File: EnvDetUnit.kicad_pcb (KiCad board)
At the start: 2 copper layers, 36 x 10 mm, 19 parts, among them CN1 CON_GROVE, CN2 CON_GROVE, J1 Conn_01x03, J2 Conn_01x03, J3 Conn_01x02, U1 S89431

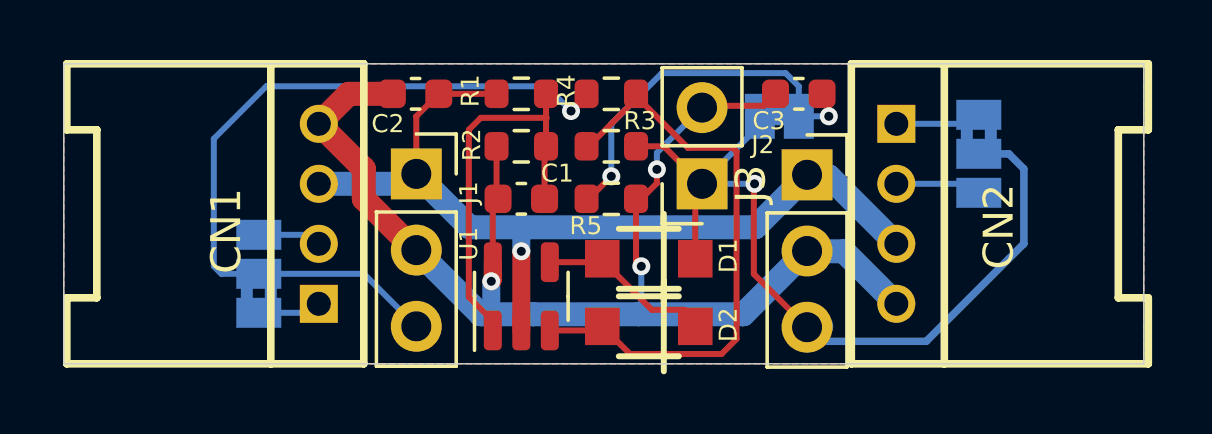
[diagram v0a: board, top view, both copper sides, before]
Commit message: update PCB data
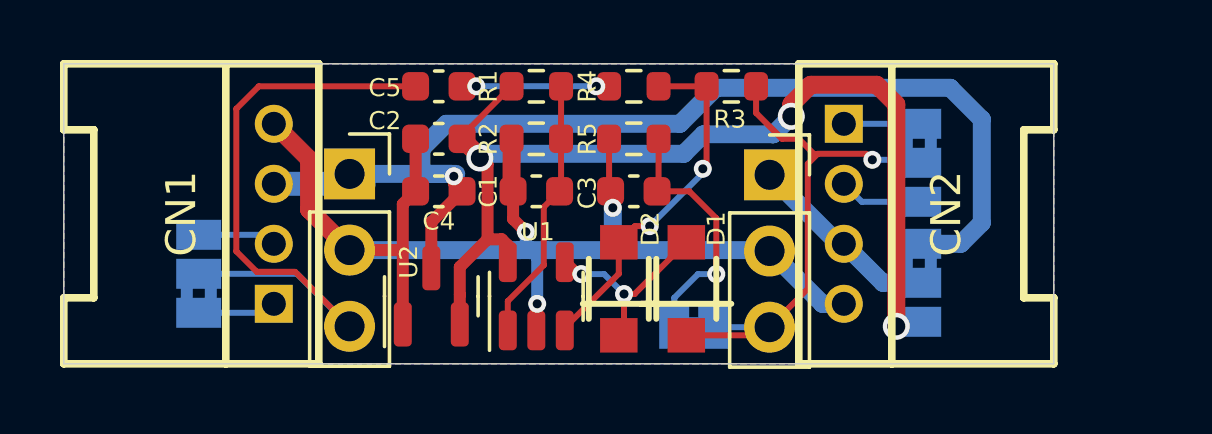
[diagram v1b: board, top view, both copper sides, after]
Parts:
- removed J3: Conn_01x02, Connector_PinSocket_2.54mm:PinSocket_1x02_P2.54mm_Vertical
- added C4: 0.1u, Capacitor_SMD:C_0603_1608Metric, F.Cu at (12.5, 4.25)
- added C5: 10u, Capacitor_SMD:C_0603_1608Metric, F.Cu at (12.5, 0.75)
- added JP4: SolderJumper_3_Bridged12, Jumper:SolderJumper-3_P1.3mm_Bridged2Bar12_Pad1.0x1.5mm_NumberLabels, B.Cu at (28.5, 7.30)
- added U2: LDO_3p_GOI, Package_TO_SOT_SMD:SOT-23, F.Cu at (12.2, 7.75)
- R5: value 1k -> 1M
- moved JP3 7.56 mm to (21.0, 8.75), turned to 0 degrees
- moved C3 6.39 mm to (19.0, 4.25)
- moved R3 4.47 mm to (22.2, 0.75)
- moved J1 2.22 mm to (9.53, 3.67)
- moved R5 2.14 mm to (19.0, 2.50), turned to 0 degrees
- moved JP2 2.02 mm to (28.5, 3.30)
- moved JP1 2.00 mm to (4.50, 7.00)
- moved CN2 1.75 mm to (26.0, 5.00)
- moved C2 1.69 mm to (12.5, 2.50)
- moved D1 1.60 mm to (20.8, 7.50), turned to -90 degrees
- moved D2 1.60 mm to (18.5, 7.50), turned to -90 degrees
- moved CN1 1.50 mm to (7.00, 5.00)
- moved J2 1.25 mm to (23.5, 3.70)
- moved R4 0.79 mm to (19.0, 0.75)
- moved C1 0.56 mm to (15.8, 4.25)
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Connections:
- C2 pad 1: +5V -> +3V3
- CN2 pad 3: +5V -> Net-(CN2-Pad3)
- J2 pad 1: +5V -> Net-(CN2-Pad3)
- R1 pad 1: +5V -> +3V3
- R4 pad 1: /Ain -> Net-(C5-Pad2)
- U1 pad 2: +5V -> GND
- U1 pad 5: GND -> +3V3
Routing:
- net +3V3: track 0.00 -> 35.2 mm, vias 0 -> 3
- net /Aout: track 29.3 -> 18.6 mm
- net +5V: track 29.7 -> 37.7 mm
- net Net-(D2-PadA): track 19.8 -> 12.0 mm, vias 0 -> 2
- net Net-(CN2-Pad3): track 0.00 -> 6.51 mm
- net Net-(C5-Pad2): track 0.00 -> 4.90 mm, vias 0 -> 2
- net /Vref: track 13.4 -> 8.87 mm
- net Net-(C3-Pad1): track 12.9 -> 8.65 mm, vias 2 -> 1
- net /Ain: track 25.6 -> 21.6 mm, vias 1 -> 0
- net GND: track 43.1 -> 41.4 mm
- net Net-(D1-PadA): track 6.14 -> 7.19 mm, vias 0 -> 2
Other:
- board size 36 x 10 mm -> 33 x 10 mm
- board text added: "+"
- board text added: "G"
